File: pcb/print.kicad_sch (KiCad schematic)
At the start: 15 parts, among them P1 USB_C_Plug, U1 CH340C, U2 ATtiny85-20S

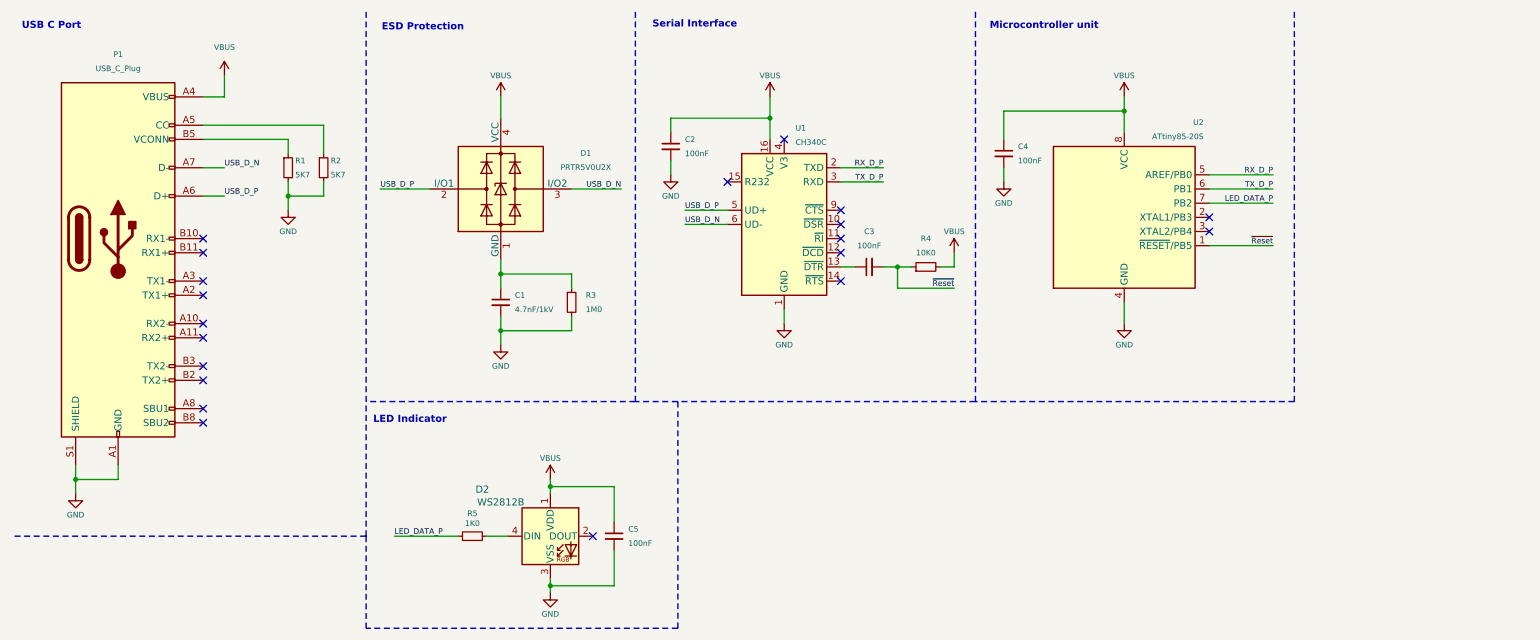
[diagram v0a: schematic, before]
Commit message: First production update.
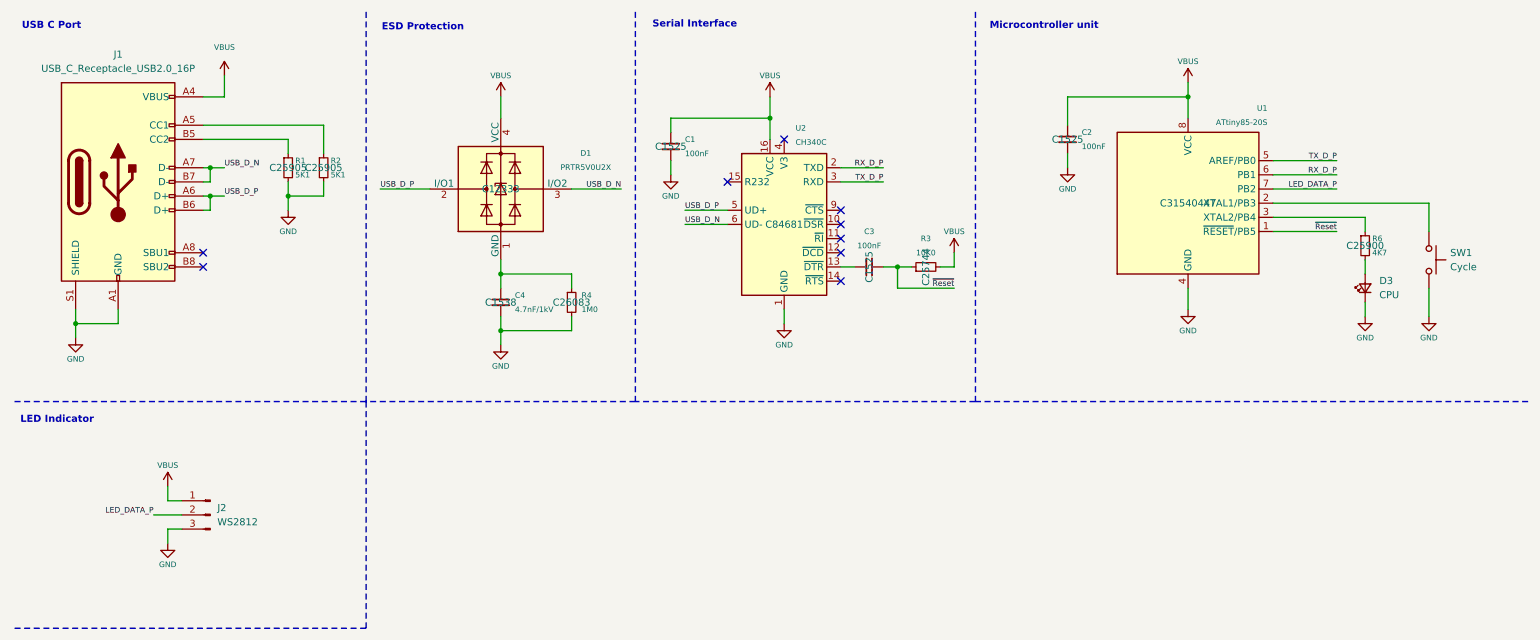
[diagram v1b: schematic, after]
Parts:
- removed C5: 100nF, symbol Device:C_Small
- removed D2: WS2812B, LED_SMD:LED_WS2812B_PLCC4_5.0x5.0mm_P3.2mm, symbol LED:WS2812B
- removed P1: USB_C_Plug, symbol Connector:USB_C_Plug
- removed R5: 1K0, symbol Device:R_Small
- added D3: CPU, Diode_SMD:D_0603_1608Metric, symbol Device:LED_Small
- added J1: USB_C_Receptacle_USB2.0_16P, Connector_USB:USB_C_Receptacle_GCT_USB4105-xx-A_16P_TopMnt_Horizontal, symbol Connector:USB_C_Receptacle_USB2.0_16P
- added J2: WS2812, Connector_PinHeader_2.54mm:PinHeader_1x03_P2.54mm_Vertical, symbol Connector:Conn_01x03_Pin
- added R6: 4K7, Resistor_SMD:R_0402_1005Metric, symbol Device:R_Small
- added SW1: Cycle, Button_Switch_THT:SW_PUSH_6mm_H4.3mm, symbol Switch:SW_Omron_B3FS
- C1: renamed from C2; footprint (none) -> Capacitor_SMD:C_0402_1005Metric; LCSC (none) -> C1525
- C2: renamed from C4; footprint (none) -> Capacitor_SMD:C_0402_1005Metric; LCSC (none) -> C1525
- C3: footprint (none) -> Capacitor_SMD:C_0402_1005Metric; LCSC (none) -> C1525
- C4: renamed from C1; footprint (none) -> Capacitor_SMD:C_0402_1005Metric; LCSC (none) -> C1538
- D1: LCSC (none) -> C12333
- R1, R2: value 5K7 -> 5K1; footprint (none) -> Resistor_SMD:R_0402_1005Metric; LCSC (none) -> C25905
- R3: renamed from R4; footprint (none) -> Resistor_SMD:R_0402_1005Metric; LCSC (none) -> C25744
- R4: renamed from R3; footprint (none) -> Resistor_SMD:R_0402_1005Metric; LCSC (none) -> C26083
- U1: renamed from U2; LCSC (none) -> C31540447
- U2: renamed from U1; LCSC (none) -> C84681
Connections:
- net GND: now also D3.1 (K), J1.A1 (GND), J1.A12 (GND), J1.B1 (GND), J1.B12 (GND), J1.S1 (SHIELD), J2.3 (Pin_3), SW1.2
- net LED_DATA_P: now also J2.2 (Pin_2)
- net RX_D_P: now also U1.6 (PB1); no longer U1.5 (AREF/PB0)
- net TX_D_P: now also U1.5 (AREF/PB0); no longer U1.6 (PB1)
- net USB_D_N: now also J1.A7 (D-), J1.B7 (D-)
- net USB_D_P: now also J1.A6 (D+), J1.B6 (D+)
- net VBUS: now also J1.A4 (VBUS), J1.A9 (VBUS), J1.B4 (VBUS), J1.B9 (VBUS), J2.1 (Pin_1)
- net at R2.1: now also J1.A5 (CC1)
- net at R1.1: now also J1.B5 (CC2)
- net at U1.2 (XTAL1/PB3): now also SW1.1
- net at U1.3 (XTAL2/PB4): now also R6.1
- new net: D3.2 (A), R6.2
- no-connect marks 20 -> 9
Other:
- title: New Project -> Do Not Disturb Indicator
- moved on the sheet: C2, U1
